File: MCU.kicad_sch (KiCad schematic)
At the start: 27 parts, among them IC1 ESP32-S3FN8, IC2 LY68L6400SLIT, J1 USB_C_Receptacle_USB2.0, SW1 SW_SPST, SW2 SW_SPST, U1 ADP7182AUJZ-3.3, Y1 40MHz

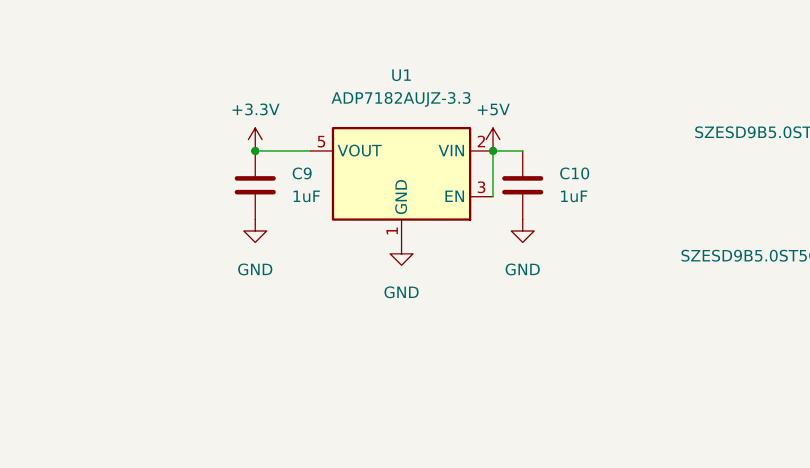
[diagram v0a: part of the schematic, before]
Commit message: ?
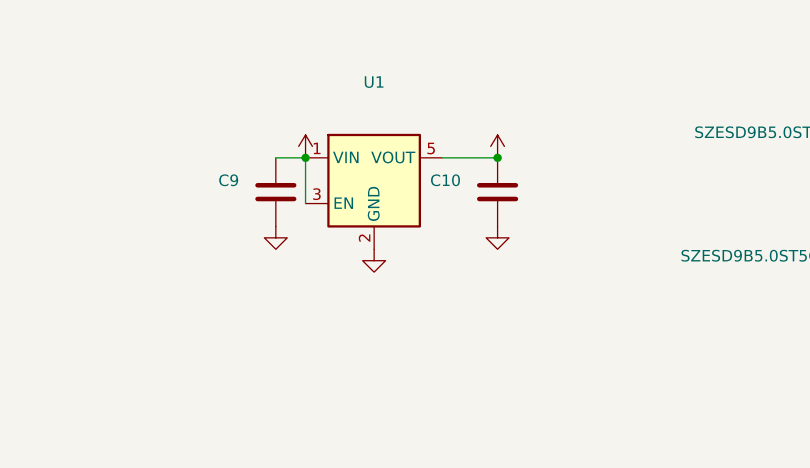
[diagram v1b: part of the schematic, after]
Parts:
- removed U1: ADP7182AUJZ-3.3, Package_TO_SOT_SMD:TSOT-23-5, symbol Regulator_Linear:ADP7182AUJZ-3.3
- added U1: (no value), symbol Regulator_Linear:NCP163ASN330T1G
- C10, C9: value 1uF -> (none); footprint Capacitor_SMD:C_0402_1005Metric -> (none)
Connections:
- net +3.3V: now also C10.1, U1.5 (VOUT); no longer C9.1
- net +5V: now also C9.1, U1.1 (VIN), U1.3 (EN); no longer C10.1
- net GND: now also U1.2 (GND)

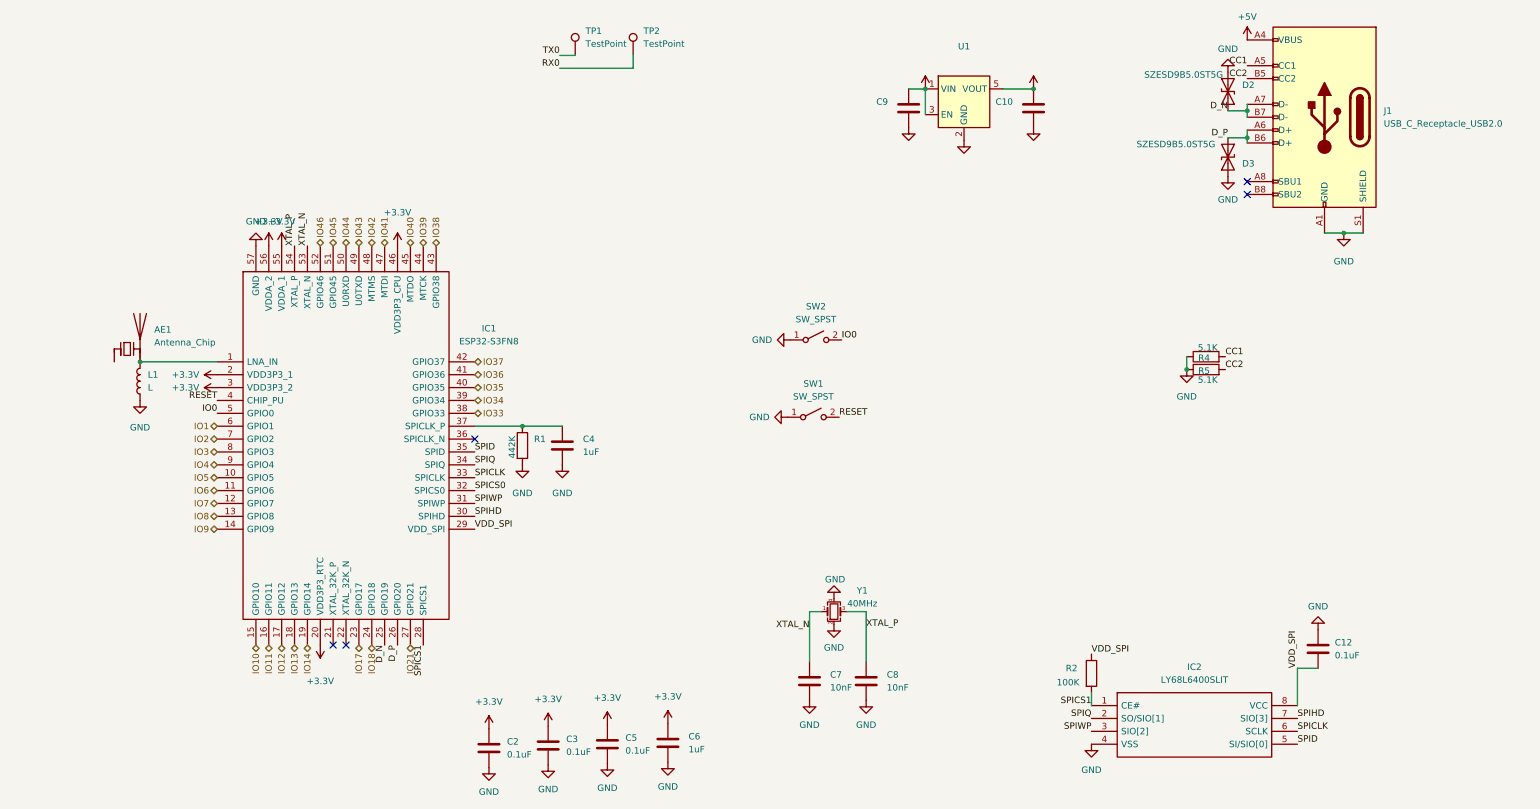
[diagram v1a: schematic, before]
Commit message: init routing done
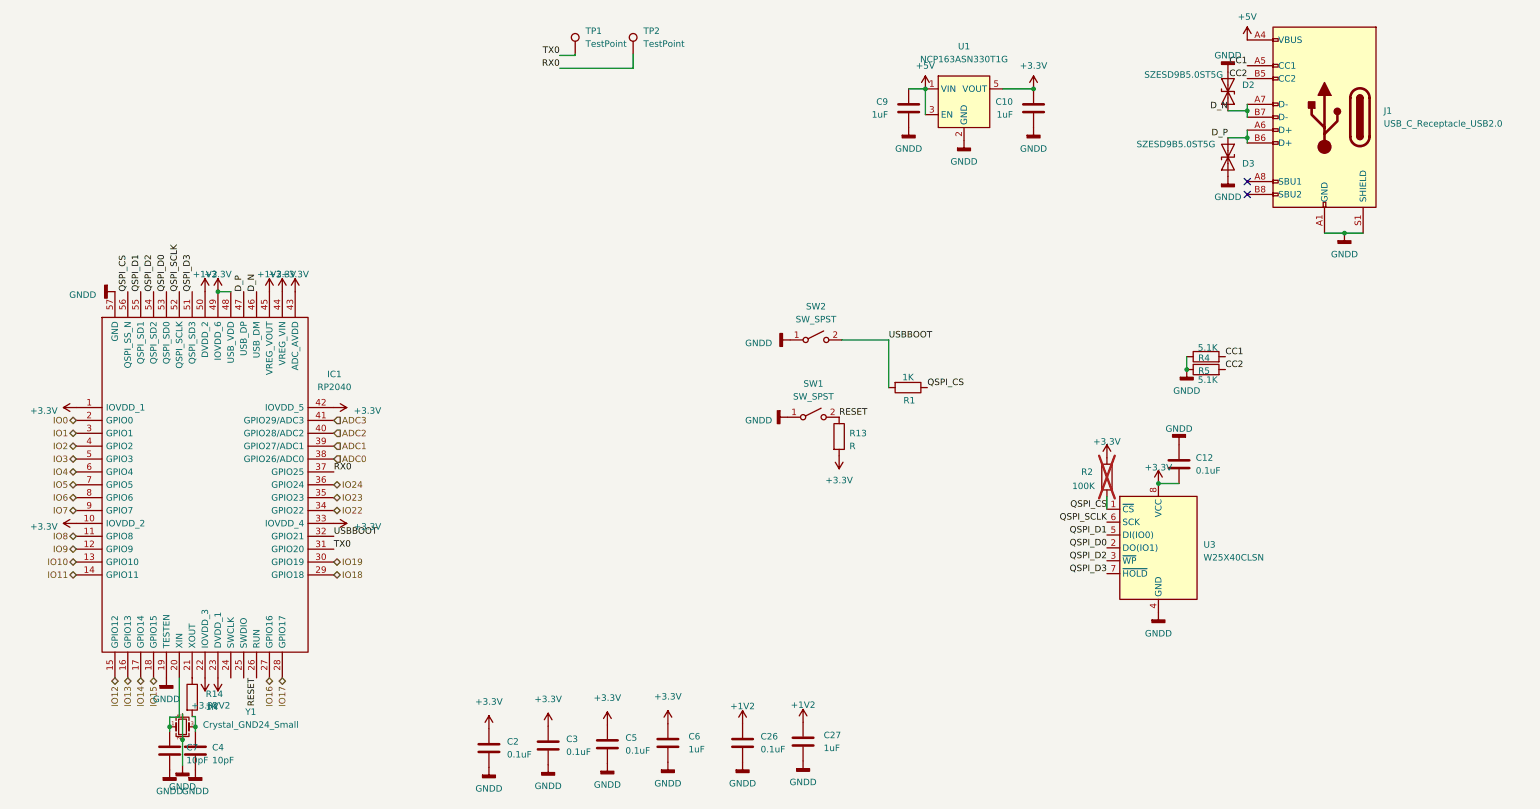
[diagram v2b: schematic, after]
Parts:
- removed AE1: Antenna_Chip, 2450AT43F0100:ANTC6020X130N, symbol Device:Antenna_Chip
- removed C8: 10nF, Capacitor_SMD:C_0402_1005Metric, symbol Device:C
- removed IC1: ESP32-S3FN8, esp32-s3:QFN40P700X700X90-57N-D, symbol ESP32-S3FN8:ESP32-S3FN8
- removed IC2: LY68L6400SLIT, LY68L6400SLIT:SOIC127P600X175-8N, symbol LY68L6400SLIT:LY68L6400SLIT
- removed L1: L, Inductor_SMD:L_0402_1005Metric, symbol Device:L
- added C26: 0.1uF, Capacitor_SMD:C_0402_1005Metric, symbol Device:C
- added C27: 1uF, Capacitor_SMD:C_0402_1005Metric, symbol Device:C
- added IC1: RP2040, RP2040:QFN40P700X700X90-57N-D, symbol RP2040:RP2040
- added R13: R, Resistor_SMD:R_0402_1005Metric, symbol Device:R
- added R14: 1K, Resistor_SMD:R_0402_1005Metric, symbol Device:R
- added U3: W25X40CLSN, Package_SO:SOIC-8_3.9x4.9mm_P1.27mm, symbol Memory_Flash:W25X40CLSN
- C10, C9: value (none) -> 1uF; footprint (none) -> Capacitor_SMD:C_0402_1005Metric
- C4: value 1uF -> 10pF
- C7: value 10nF -> 10pF
- R1: value 442K -> 1K
- R2: now not fitted
- U1: value (none) -> NCP163ASN330T1G; footprint (none) -> Package_TO_SOT_SMD:SOT-23-5
- Y1: value 40MHz -> Crystal_GND24_Small; footprint Crystal:Crystal_SMD_2016-4Pin_2.0x1.6mm -> Crystal:Crystal_SMD_2520-4Pin_2.5x2.0mm
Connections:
- net VDD_SPI is gone; now on net +3.3V: C12.2, R2.1
- net XTAL_P is gone; now on an unnamed net: Y1.3
- net +3.3V: now also IC1.1 (IOVDD_1), IC1.10 (IOVDD_2), IC1.22 (IOVDD_3), IC1.33 (IOVDD_4), IC1.42 (IOVDD_5), IC1.43 (ADC_AVDD), IC1.44 (VREG_VIN), IC1.48 (USB_VDD), IC1.49 (IOVDD_6), R13.2, U3.8 (VCC)
- net D_N: now also IC1.46 (USB_DM)
- net D_P: now also IC1.47 (USB_DP)
- net IO0: now also IC1.2 (GPIO0); no longer SW2.2 (B)
- net IO1: now also IC1.3 (GPIO1)
- net IO10: now also IC1.13 (GPIO10)
- net IO11: now also IC1.14 (GPIO11)
- net IO12: now also IC1.15 (GPIO12)
- net IO13: now also IC1.16 (GPIO13)
- net IO14: now also IC1.17 (GPIO14)
- net IO17: now also IC1.28 (GPIO17)
- net IO18: now also IC1.29 (GPIO18)
- net IO2: now also IC1.4 (GPIO2)
- net IO3: now also IC1.5 (GPIO3)
- net IO4: now also IC1.6 (GPIO4)
- net IO5: now also IC1.7 (GPIO5)
- net IO6: now also IC1.8 (GPIO6)
- net IO7: now also IC1.9 (GPIO7)
- net IO8: now also IC1.11 (GPIO8)
- net IO9: now also IC1.12 (GPIO9)
- net RESET: now also IC1.26 (RUN), R13.1
- net RX0: now also IC1.37 (GPIO25)
- net TX0: now also IC1.31 (GPIO20)
- net at C4.1: now also R14.2; no longer R1.1
- net GND renamed GNDD
- net GNDD: now also C26.2, C27.2, IC1.19 (TESTEN), IC1.57 (GND), U3.4 (GND); no longer R1.2
- net SPICS1 renamed QSPI_CS
- net QSPI_CS: now also R1.1, IC1.56 (QSPI_SS_N), U3.1 (~{CS})
- net XTAL_N: no longer names the net of C7.1, Y1.1
- net XTAL_N: now also IC1.20 (XIN)
- new net: IC1.21 (XOUT), R14.1
- new net +1V2: C26.1, C27.1, IC1.23 (DVDD_1), IC1.45 (VREG_VOUT), IC1.50 (DVDD_2)
- new net ADC0: IC1.38 (GPIO26/ADC0)
- new net ADC1: IC1.39 (GPIO27/ADC1)
- new net ADC2: IC1.40 (GPIO28/ADC2)
- new net ADC3: IC1.41 (GPIO29/ADC3)
- new net IO15: IC1.18 (GPIO15)
- new net IO16: IC1.27 (GPIO16)
- new net IO19: IC1.30 (GPIO19)
- new net IO22: IC1.34 (GPIO22)
- new net IO23: IC1.35 (GPIO23)
- new net IO24: IC1.36 (GPIO24)
- new net QSPI_D0: IC1.53 (QSPI_SD0), U3.2 (DO(IO1))
- new net QSPI_D1: IC1.55 (QSPI_SD1), U3.5 (DI(IO0))
- new net QSPI_D2: IC1.54 (QSPI_SD2), U3.3 (~{WP})
- new net QSPI_D3: IC1.51 (QSPI_SD3), U3.7 (~{HOLD})
- new net QSPI_SCLK: IC1.52 (QSPI_SCLK), U3.6 (SCK)
- new net USBBOOT: IC1.32 (GPIO21), R1.2, SW2.2 (B)
- no-connect marks 5 -> 2
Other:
- moved on the sheet: C12

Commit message: designed
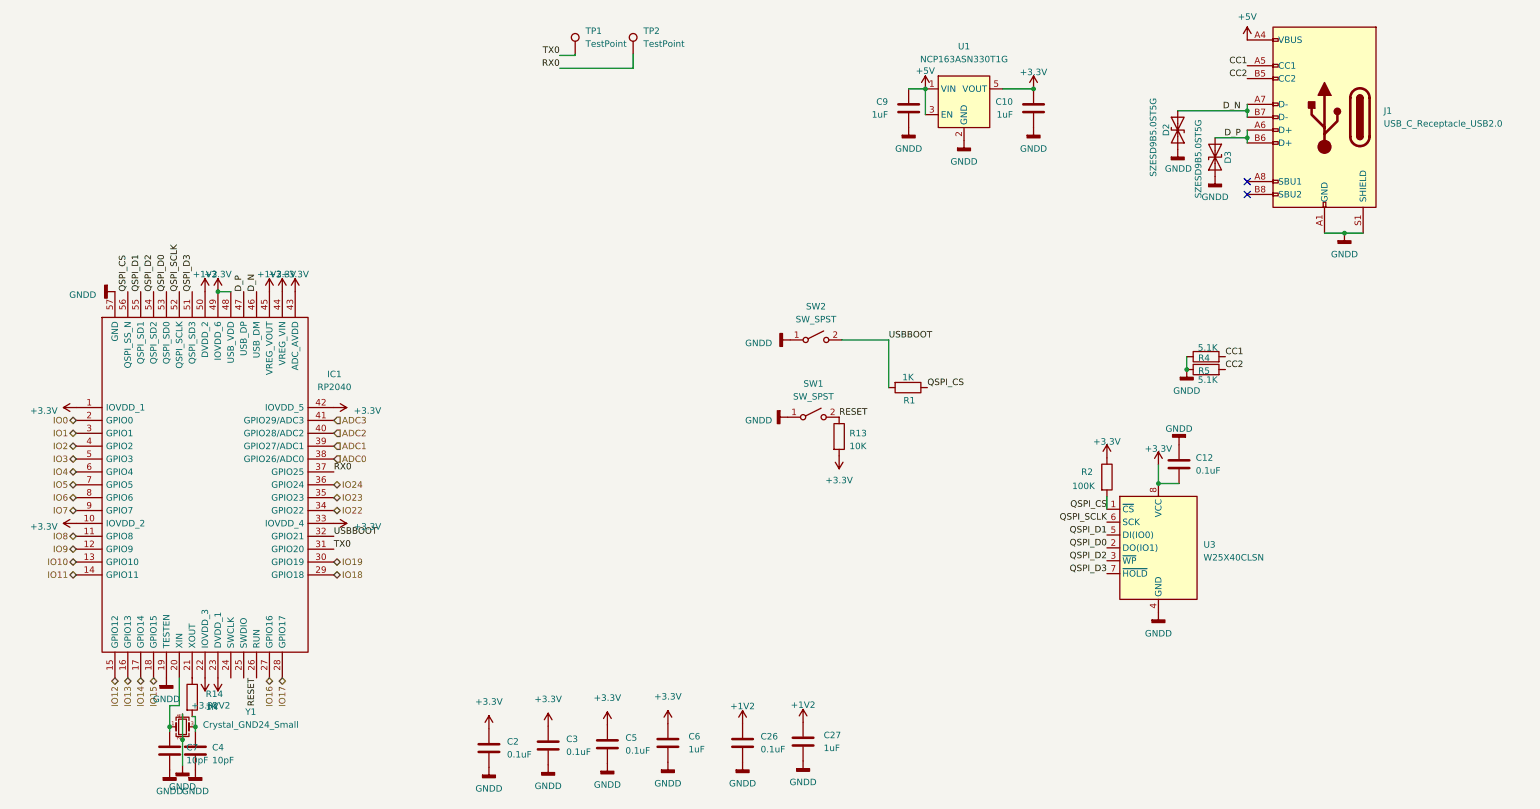
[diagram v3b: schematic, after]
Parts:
- R13: value R -> 10K
- R2: now fitted
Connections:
- net D_N: now also D2.2 (A2); no longer D2.1 (A1)
- net GNDD: now also D2.1 (A1); no longer D2.2 (A2)
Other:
- moved on the sheet: D2, D3
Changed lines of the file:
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@@
-(kicad_sch (version 20221206) (generator eeschema)
+(kicad_sch (version 20230121) (generator eeschema)
   (paper "A4")
   (junction (at 216.662 28.194) (diameter 0) (color 0 0 0 0)
@@
   (junction (at 51.308 154.051) (diameter 0) (color 0 0 0 0)
   )
+  (junction (at 195.326 28.194) (diameter 0) (color 0 0 0 0)
+  )
   (junction (at 258.826 32.512) (diameter 0) (color 0 0 0 0)
-  )
-  (junction (at 195.326 28.194) (diameter 0) (color 0 0 0 0)
   )
   (junction (at 258.826 37.846) (diameter 0) (color 0 0 0 0)
@@
     (stroke (width 0) (type default))
   )
-  (wire (pts (xy 48.133 152.146) (xy 46.228 152.146))
+  (wire (pts (xy 48.133 149.86) (xy 46.228 149.86))
     (stroke (width 0) (type default))
   )
@@
     (stroke (width 0) (type default))
   )
-  (wire (pts (xy 255.016 37.846) (xy 258.826 37.846))
+  (wire (pts (xy 252.476 37.846) (xy 258.826 37.846))
     (stroke (width 0) (type default))
   )
@@
     (stroke (width 0) (type default))
   )
+  (wire (pts (xy 241.3 102.362) (xy 241.3 106.045))
+    (stroke (width 0) (type default))
+  )
   (wire (pts (xy 258.826 31.242) (xy 258.826 32.512))
     (stroke (width 0) (type default))
@@
     (stroke (width 0) (type default))
   )
-  (wire (pts (xy 255.016 32.512) (xy 258.826 32.512))
-    (stroke (width 0) (type default))
-  )
   (wire (pts (xy 195.326 28.194) (xy 195.326 33.274))
     (stroke (width 0) (type default))
@@
     (stroke (width 0) (type default))
   )
+  (wire (pts (xy 245.11 32.512) (xy 258.826 32.512))
+    (stroke (width 0) (type default))
+  )
   (wire (pts (xy 48.768 156.591) (xy 48.768 161.671))
     (stroke (width 0) (type default))
   )
-  (wire (pts (xy 46.228 152.146) (xy 46.228 154.051))
-    (stroke (width 0) (type default))
-  )
   (wire (pts (xy 246.888 81.026) (xy 246.888 83.566))
     (stroke (width 0) (type default))
@@
     (stroke (width 0) (type default))
   )
-  (wire (pts (xy 48.133 144.399) (xy 48.133 152.146))
+  (wire (pts (xy 48.133 144.399) (xy 48.133 149.86))
     (stroke (width 0) (type default))
   )
   (wire (pts (xy 195.326 28.194) (xy 192.024 28.194))
+    (stroke (width 0) (type default))
+  )
+  (wire (pts (xy 46.228 149.86) (xy 46.228 154.051))
     (stroke (width 0) (type default))
   )
@@
     (effects (font (size 1.27 1.27)) (justify left bottom))
   )
-  (label "D_N" (at 255.016 32.512 180) (fields_autoplaced)
-    (effects (font (size 1.27 1.27)) (justify right bottom))
-  )
-  (label "D_P" (at 255.016 37.846 180) (fields_autoplaced)
+  (label "D_N" (at 254 32.512 0) (fields_autoplaced)
+    (effects (font (size 1.27 1.27)) (justify left bottom))
+  )
+  (label "D_P" (at 257.556 37.846 180) (fields_autoplaced)
     (effects (font (size 1.27 1.27)) (justify right bottom))
   )
@@
     )
   )
-  (symbol (lib_name "+3.3V_5") (lib_id "power:+3.3V") (at 241.3 106.045 0) (unit 1)
-    (in_bom yes) (on_board yes) (dnp no) (fields_autoplaced)
-    (property "Reference" "#PWR027" (at 241.3 109.855 0)
-      (effects (font (size 1.27 1.27)) hide)
-    )
-    (property "Value" "+3.3V" (at 241.3 102.87 0)
-      (effects (font (size 1.27 1.27)))
-    )
-    (property "Footprint" "" (at 241.3 106.045 0)
-      (effects (font (size 1.27 1.27)) hide)
-    )
-    (property "Datasheet" "" (at 241.3 106.045 0)
+  (symbol (lib_name "+3.3V_5") (lib_id "power:+3.3V") (at 241.3 102.362 0) (unit 1)
+    (in_bom yes) (on_board yes) (dnp no) (fields_autoplaced)
+    (property "Reference" "#PWR027" (at 241.3 106.172 0)
+      (effects (font (size 1.27 1.27)) hide)
+    )
+    (property "Value" "+3.3V" (at 241.3 99.187 0)
+      (effects (font (size 1.27 1.27)))
+    )
+    (property "Footprint" "" (at 241.3 102.362 0)
+      (effects (font (size 1.27 1.27)) hide)
+    )
+    (property "Datasheet" "" (at 241.3 102.362 0)
       (effects (font (size 1.27 1.27)) hide)
     )
@@
     )
   )
-  (symbol (lib_id "power:GNDD") (at 255.016 45.466 0) (unit 1)
-    (in_bom yes) (on_board yes) (dnp no) (fields_autoplaced)
-    (property "Reference" "#PWR029" (at 255.016 51.816 0)
-      (effects (font (size 1.27 1.27)) hide)
-    )
-    (property "Value" "GNDD" (at 255.016 49.53 0)
-      (effects (font (size 1.27 1.27)))
-    )
-    (property "Footprint" "" (at 255.016 45.466 0)
-      (effects (font (size 1.27 1.27)) hide)
-    )
-    (property "Datasheet" "" (at 255.016 45.466 0)
+  (symbol (lib_id "power:GNDD") (at 252.476 45.466 0) (unit 1)
+    (in_bom yes) (on_board yes) (dnp no) (fields_autoplaced)
+    (property "Reference" "#PWR029" (at 252.476 51.816 0)
+      (effects (font (size 1.27 1.27)) hide)
+    )
+    (property "Value" "GNDD" (at 252.476 49.53 0)
+      (effects (font (size 1.27 1.27)))
+    )
+    (property "Footprint" "" (at 252.476 45.466 0)
+      (effects (font (size 1.27 1.27)) hide)
+    )
+    (property "Datasheet" "" (at 252.476 45.466 0)
       (effects (font (size 1.27 1.27)) hide)
     )
@@
   )
   (symbol (lib_id "power:+5V") (at 195.326 28.194 0) (mirror y) (unit 1)
-    (in_bom yes) (on_board yes) (dnp no) (fields_autoplaced)
+    (in_bom yes) (on_board yes) (dnp no)
     (property "Reference" "#PWR0140" (at 195.326 32.004 0)
       (effects (font (size 1.27 1.27)) hide)
     )
-    (property "Value" "+5V" (at 195.326 23.622 0)
+    (property "Value" "+5V" (at 195.326 24.638 0)
       (effects (font (size 1.27 1.27)))
     )
@@
       (effects (font (size 1.27 1.27)) (justify left))
     )
-    (property "Value" "R" (at 180.34 98.679 0)
+    (property "Value" "10K" (at 180.34 98.679 0)
       (effects (font (size 1.27 1.27)) (justify left))
     )
@@
     )
   )
-  (symbol (lib_id "Diode:SZESD9B5.0ST5G") (at 255.016 41.656 90) (mirror x) (unit 1)
+  (symbol (lib_id "Diode:SZESD9B5.0ST5G") (at 252.476 41.656 90) (mirror x) (unit 1)
     (in_bom yes) (on_board yes) (dnp no)
-    (property "Reference" "D3" (at 257.81 42.9261 90)
+    (property "Reference" "D3" (at 255.016 42.926 0)
       (effects (font (size 1.27 1.27)) (justify right))
     )
-    (property "Value" "SZESD9B5.0ST5G" (at 236.982 39.116 90)
+    (property "Value" "SZESD9B5.0ST5G" (at 249.174 49.784 0)
       (effects (font (size 1.27 1.27)) (justify right))
     )
-    (property "Footprint" "Diode_SMD:D_SOD-923" (at 255.016 41.656 0)
-      (effects (font (size 1.27 1.27)) hide)
-    )
-    (property "Datasheet" "https://www.onsemi.com/pub/Collateral/ESD9B-D.PDF" (at 255.016 41.656 0)
+    (property "Footprint" "Diode_SMD:D_SOD-923" (at 252.476 41.656 0)
+      (effects (font (size 1.27 1.27)) hide)
+    )
+    (property "Datasheet" "https://www.onsemi.com/pub/Collateral/ESD9B-D.PDF" (at 252.476 41.656 0)
       (effects (font (size 1.27 1.27)) hide)
     )
@@
   )
   (symbol (lib_id "Device:R") (at 231.14 104.775 0) (unit 1)
-    (in_bom yes) (on_board yes) (dnp yes)
+    (in_bom yes) (on_board yes) (dnp no)
     (property "Reference" "R2" (at 226.06 103.759 0)
       (effects (font (size 1.27 1.27)) (justify left))
@@
   )
   (symbol (lib_id "power:+3.3V") (at 216.662 28.194 0) (mirror y) (unit 1)
-    (in_bom yes) (on_board yes) (dnp no) (fields_autoplaced)
+    (in_bom yes) (on_board yes) (dnp no)
     (property "Reference" "#PWR0138" (at 216.662 32.004 0)
       (effects (font (size 1.27 1.27)) hide)
     )
-    (property "Value" "+3.3V" (at 216.662 23.622 0)
+    (property "Value" "+3.3V" (at 216.662 24.892 0)
       (effects (font (size 1.27 1.27)))
     )
@@
     )
   )
-  (symbol (lib_id "Diode:SZESD9B5.0ST5G") (at 255.016 28.702 90) (unit 1)
+  (symbol (lib_id "Diode:SZESD9B5.0ST5G") (at 245.11 36.322 90) (unit 1)
     (in_bom yes) (on_board yes) (dnp no)
-    (property "Reference" "D2" (at 257.81 27.4319 90)
+    (property "Reference" "D2" (at 242.824 35.052 0)
       (effects (font (size 1.27 1.27)) (justify right))
     )
-    (property "Value" "SZESD9B5.0ST5G" (at 238.506 25.4 90)
+    (property "Value" "SZESD9B5.0ST5G" (at 240.284 29.972 0)
       (effects (font (size 1.27 1.27)) (justify right))
     )
-    (property "Footprint" "Diode_SMD:D_SOD-923" (at 255.016 28.702 0)
-      (effects (font (size 1.27 1.27)) hide)
-    )
-    (property "Datasheet" "https://www.onsemi.com/pub/Collateral/ESD9B-D.PDF" (at 255.016 28.702 0)
+    (property "Footprint" "Diode_SMD:D_SOD-923" (at 245.11 36.322 0)
+      (effects (font (size 1.27 1.27)) hide)
+    )
+    (property "Datasheet" "https://www.onsemi.com/pub/Collateral/ESD9B-D.PDF" (at 245.11 36.322 0)
       (effects (font (size 1.27 1.27)) hide)
     )
@@
     )
   )
-  (symbol (lib_id "power:GNDD") (at 255.016 24.892 180) (unit 1)
-    (in_bom yes) (on_board yes) (dnp no) (fields_autoplaced)
-    (property "Reference" "#PWR035" (at 255.016 18.542 0)
-      (effects (font (size 1.27 1.27)) hide)
-    )
-    (property "Value" "GNDD" (at 255.016 21.59 0)
-      (effects (font (size 1.27 1.27)))
-    )
-    (property "Footprint" "" (at 255.016 24.892 0)
-      (effects (font (size 1.27 1.27)) hide)
-    )
-    (property "Datasheet" "" (at 255.016 24.892 0)
-      (effects (font (size 1.27 1.27)) hide)
-    )
+  (symbol (lib_id "power:GNDD") (at 245.11 40.132 0) (unit 1)
+    (in_bom yes) (on_board yes) (dnp no)
+    (property "Reference" "#PWR035" (at 245.11 46.482 0)
+      (effects (font (size 1.27 1.27)) hide)
+    )
+    (property "Value" "GNDD" (at 242.57 43.942 0)
+      (effects (font (size 1.27 1.27)) (justify left))
+    )
+    (property "Footprint" "" (at 245.11 40.132 0)
+      (effects (font (size 1.27 1.27)) hide)
+    )
+    (property "Datasheet" "" (at 245.11 40.132 0)
+      (effects (font (size 1.27 1.27)) hide)
+    )
